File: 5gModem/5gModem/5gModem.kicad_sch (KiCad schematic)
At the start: 8 parts, among them J1 USB_C_Receptacle_PowerOnly_6P, J2 USB_C_Receptacle_USB2.0_14P

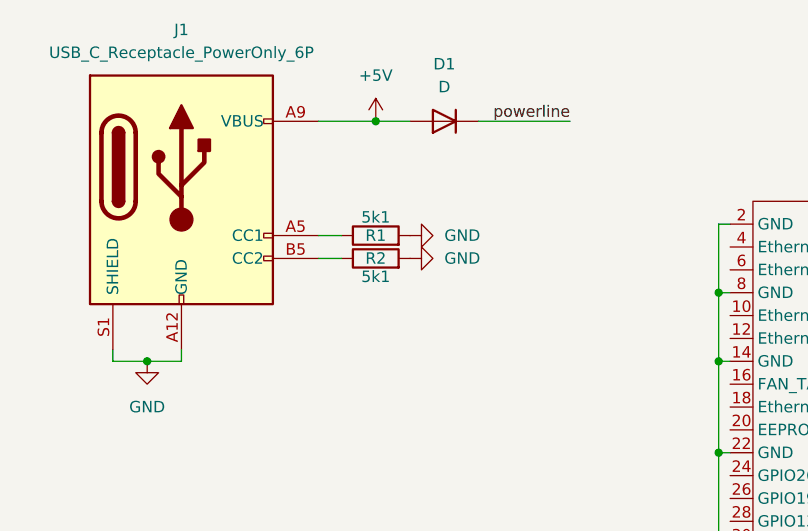
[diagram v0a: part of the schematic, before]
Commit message: Worked a little
I think its far from done but I'm proud of what I have
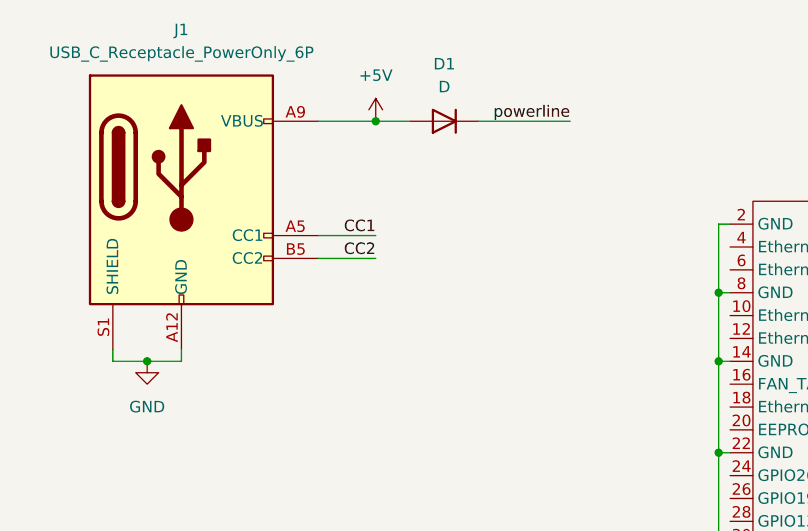
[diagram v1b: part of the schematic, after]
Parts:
- removed R1, R2: 5k1, Resistor_SMD:R_1210_3225Metric_Pad1.30x2.65mm_HandSolder, symbol Device:R
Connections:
- net CC1: now also J1.A5 (CC1)
- net CC2: now also J1.B5 (CC2)
